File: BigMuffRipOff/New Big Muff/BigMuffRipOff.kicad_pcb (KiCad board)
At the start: 4 copper layers, 50.8 x 84 mm, 92 parts, among them J1 284697-E, J2 NMJ6HFD2, J3 NMJ6HFD2, J4 2125201004, J5 PJ-007, J6 2125201004, J7 2125201004, J8 Conn_01x04, Q1 BC549, Q2 BC549, Q3 BC549, Q4 BC549, SW3 B3FS-1010P, U1 TPL0501-100DCNR, U10 R-78E3.3-0.5, U2 TPL0501-100DCNR, U3 TPL0501-100DCNR, U4 TL071HIDBVR, U5 TL071HIDBVR, U6 ADP7118AUJZ-4.5-R7, U7 TL071HIDBVR, U8 TPL0501-100DCNR, U9 STM8L152K4T6

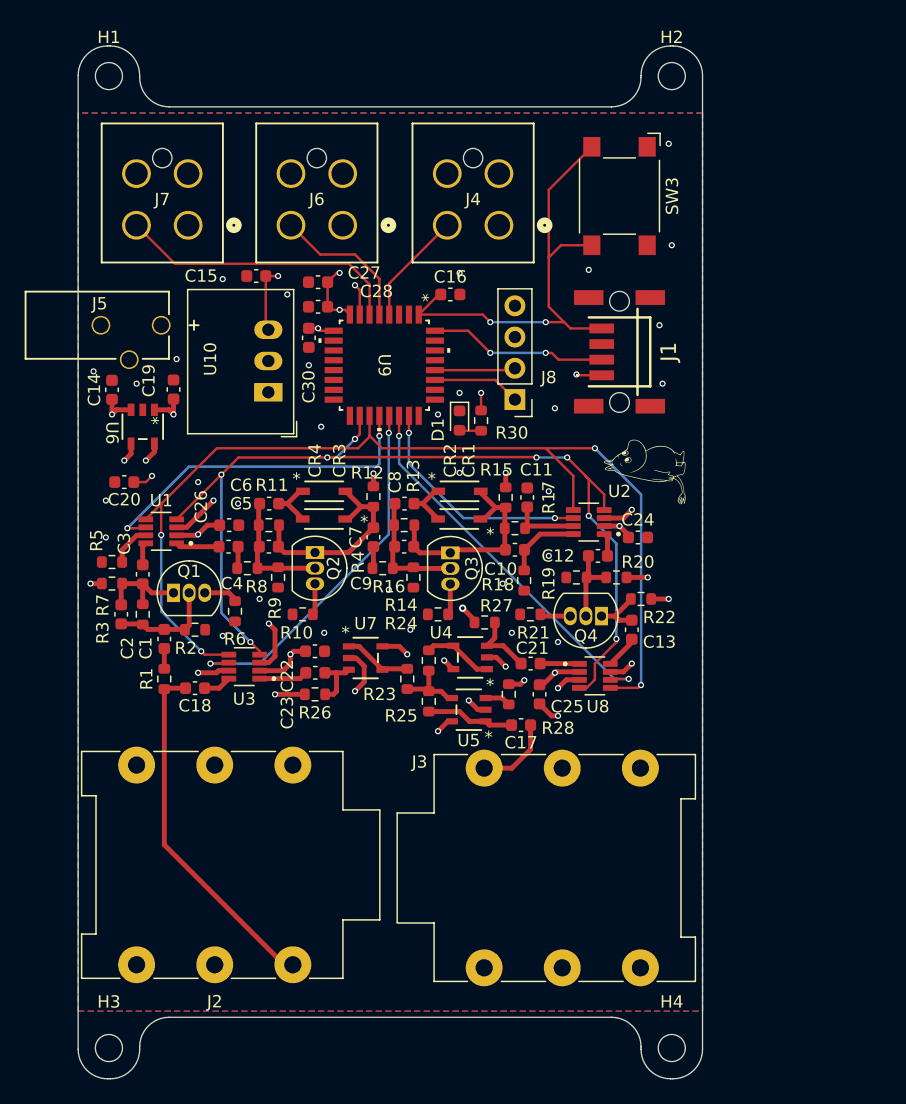
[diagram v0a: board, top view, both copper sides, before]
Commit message: new big muff completed
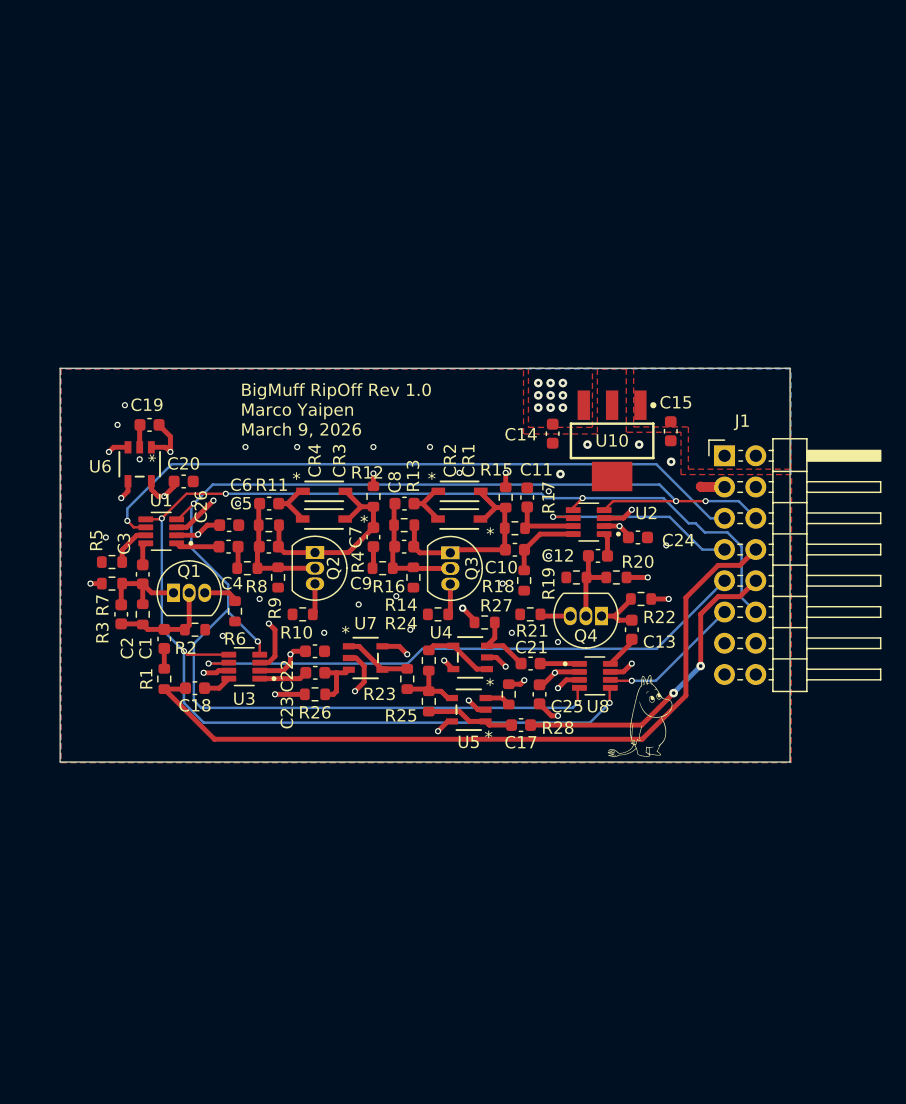
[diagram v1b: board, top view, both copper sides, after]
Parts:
- removed C16: 0.1u, Capacitor_SMD:C_0603_1608Metric
- removed C27: 10n, Capacitor_SMD:C_0603_1608Metric
- removed C28: 100n, Capacitor_SMD:C_0603_1608Metric
- removed C30: 1u, Capacitor_SMD:C_0603_1608Metric
- removed D1: LED, LED_SMD:LED_0603_1608Metric
- removed the G*** at (148.8, 83.3)
- removed H1, H2, H3, H4: MountingHole, MountingHole:MountingHole_2.2mm_M2
- removed J2, J3: NMJ6HFD2, Connector_Audio:Jack_6.35mm_Neutrik_NMJ6HFD2_Horizontal
- removed J4, J6, J7: 2125201004, 284867-E-footprint:CONN_2125200001-SD_04_MOL
- removed J5: PJ-007, 284867-E-footprint:CONN_PJ-007_SSD
- removed J8: Conn_01x04, Connector_PinHeader_2.54mm:PinHeader_1x04_P2.54mm_Vertical
- removed R30: 270, Resistor_SMD:R_0603_1608Metric
- removed SW3: B3FS-1010P, Button_Switch_SMD:SW_SPST_Omron_B3FS-101xP
- removed U9: STM8L152K4T6, 284867-E-footprint:LQFP-32
- C14: value 10u -> 22u
- C15: value 10u -> 0.47u
- J1: value 284697-E -> Conn_02x08_Odd_Even; footprint 284867-E-footprint:284697E -> Connector_PinHeader_2.54mm:PinHeader_2x08_P2.54mm_Horizontal
- U10: value R-78E3.3-0.5 -> LM2940IMP-9.0/NOPB; footprint Converter_DCDC:Converter_DCDC_RECOM_R-78E-0.5_THT -> GTSR_KiCAD_Footprints:DCY0004A_N
- moved C14 36.0 mm to (163.6, 76.3), turned to -90 degrees
- moved C15 36.0 mm to (173.2, 76.1), turned to -90 degrees
- moved U10 28.2 mm to (168.4, 76.9), turned to -90 degrees
- moved G*** 19.7 mm to (170.6, 99.2), turned to 0 degrees
- moved J1 12.0 mm to (177.5, 78.1), turned to 0 degrees
- moved C20 4.83 mm to (133.6, 80.2), turned to 0 degrees
- moved C19 3.47 mm to (130.8, 75.6), turned to 180 degrees
- moved U6 3.06 mm to (130.0, 78.8)
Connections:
- C15 pad 1: 3.3V -> 12V
- C17 pad 1: /Effect Stage/output_signal -> /GUITAR_OUT
- C18 pad 2: /Effect Stage/input_signal -> /GUITAR_IN
- J1 pad 1: 3.3V -> 12V
- J1 pad 2: /MCU/SWIM -> 12V
- J1 pad 4: /MCU/RST -> GND
- J1 pad 5: GND -> /CS2
- J1 pad 6: GND -> /SPI_CLK
- J1 pad 7: GND -> /CS1
- J1 pad 8: GND -> /GUITAR_IN
- R1 pad 1: /Effect Stage/input_signal -> /GUITAR_IN
- U1 pad 4: /Effect Stage/SPI_CLK -> /SPI_CLK
- U1 pad 5: /Effect Stage/SPI_MOSI -> /MOSI
- U1 pad 6: /Effect Stage/CS_1 -> /CS2
- U10 pad 1: 9V -> 12V
- U10 pad 3: 3.3V -> 9V
- U2 pad 4: /Effect Stage/SPI_CLK -> /SPI_CLK
- U2 pad 5: /Effect Stage/SPI_MOSI -> /MOSI
- U2 pad 6: /Effect Stage/CS_2 -> /CS1
- U3 pad 4: /Effect Stage/SPI_CLK -> /SPI_CLK
- U3 pad 5: /Effect Stage/SPI_MOSI -> /MOSI
- U3 pad 6: /Effect Stage/CS_4 -> /CS3
- U8 pad 4: /Effect Stage/SPI_CLK -> /SPI_CLK
- U8 pad 5: /Effect Stage/SPI_MOSI -> /MOSI
- U8 pad 6: /Effect Stage/CS_3 -> /CS0
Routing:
- net /MOSI: track 0.00 -> 114.8 mm, vias 0 -> 5
- net /SPI_CLK: track 0.00 -> 111.6 mm, vias 0 -> 5
- net /Effect Stage/SPI_MOSI: track 86.5 -> 0.00 mm, vias 4 -> 0
- net /Effect Stage/SPI_CLK: track 80.1 -> 0.00 mm, vias 8 -> 0
- net /GUITAR_IN: track 0.00 -> 62.6 mm
- net /CS2: track 0.00 -> 54.6 mm, vias 0 -> 1
- net /CS3: track 0.00 -> 46.4 mm, vias 0 -> 1
- net /MCU/RST: track 38.9 -> 0.00 mm, vias 2 -> 0
- net /Effect Stage/CS_3: track 31.3 -> 0.00 mm, vias 2 -> 0
- net /Effect Stage/CS_4: track 30.0 -> 0.00 mm, vias 2 -> 0
- net /Effect Stage/input_signal: track 28.2 -> 0.00 mm
- net /Effect Stage/CS_1: track 28.1 -> 0.00 mm, vias 2 -> 0
- net /GUITAR_OUT: track 0.00 -> 25.6 mm, vias 0 -> 2
- net /MCU/Pot_3: track 23.4 -> 0.00 mm
- net /Effect Stage/CS_2: track 19.1 -> 0.00 mm, vias 2 -> 0
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- added copper zone on F.Cu, net 12V
- added copper zone on F.Cu, net 9V
- removed copper zone on In2.Cu, net 3.3V
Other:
- board size 50.8 x 84 mm -> 59.3 x 32 mm
- board text added: "BigMuff RipOff Rev 1.0 Marco Yaipen March 9, 2026"
- board text removed: "Marco Yaipen BigMuff RipOff Rev 1.0 February 14, 2026"
